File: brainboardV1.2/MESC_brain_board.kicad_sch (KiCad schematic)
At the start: 17 parts, among them J1 Conn_01x18, J2 Conn_01x04, Q1 my_BC337, U2 TJA1050T/CM,118, U2 Teensy4.0

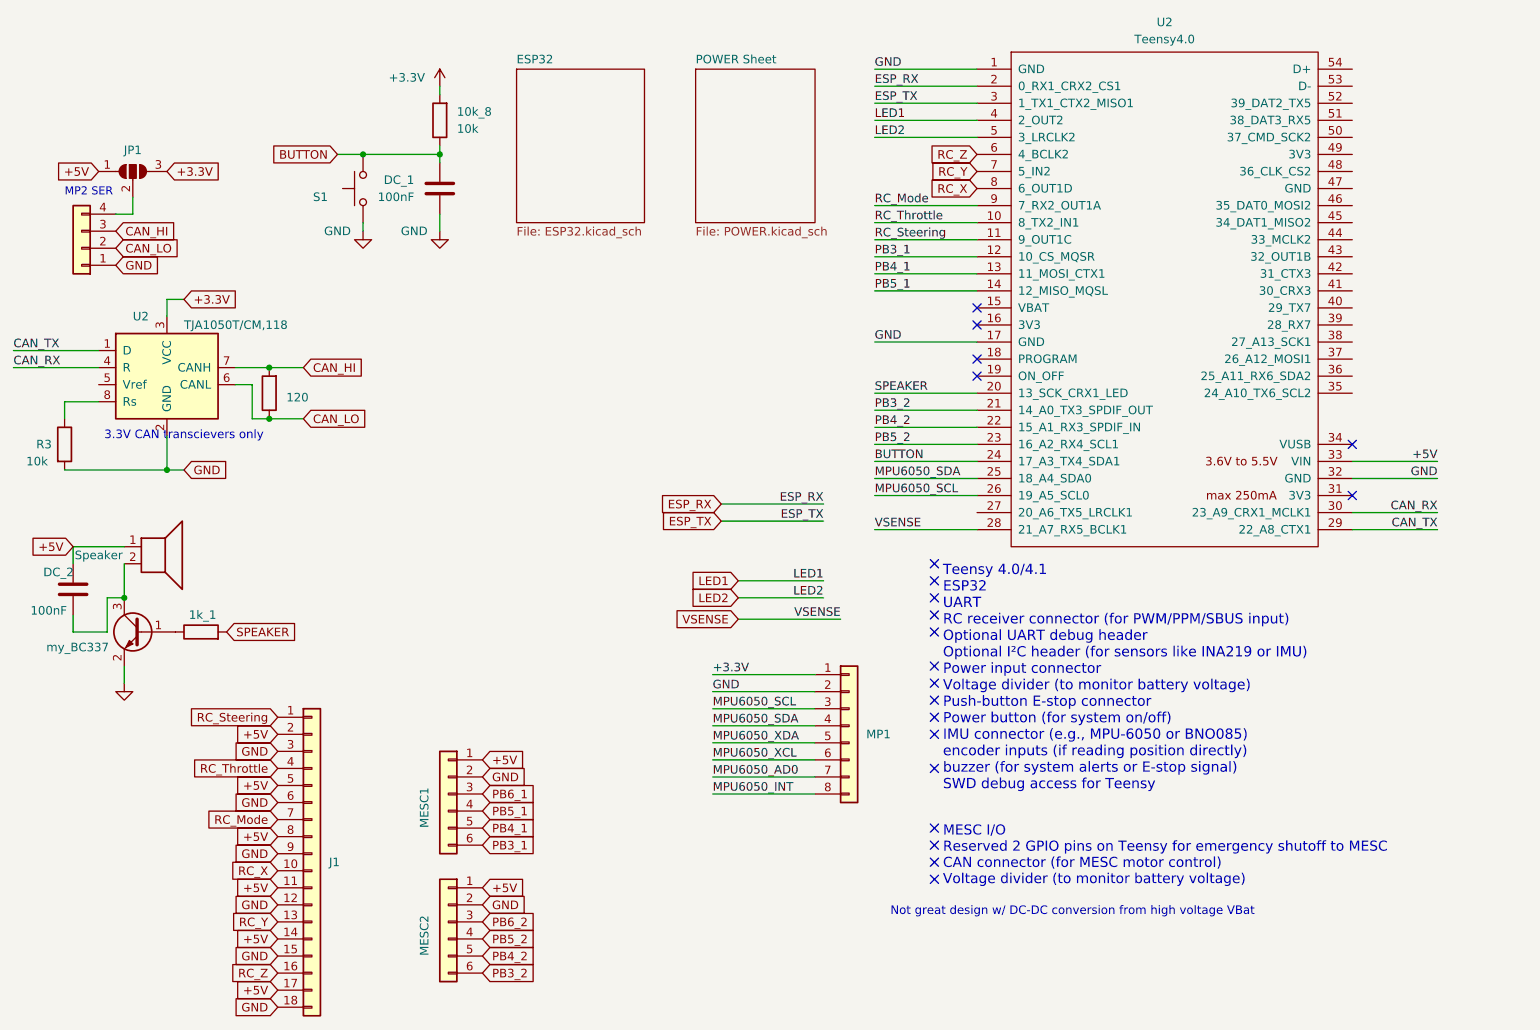
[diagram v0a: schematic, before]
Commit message: finalizing brain board v1.2
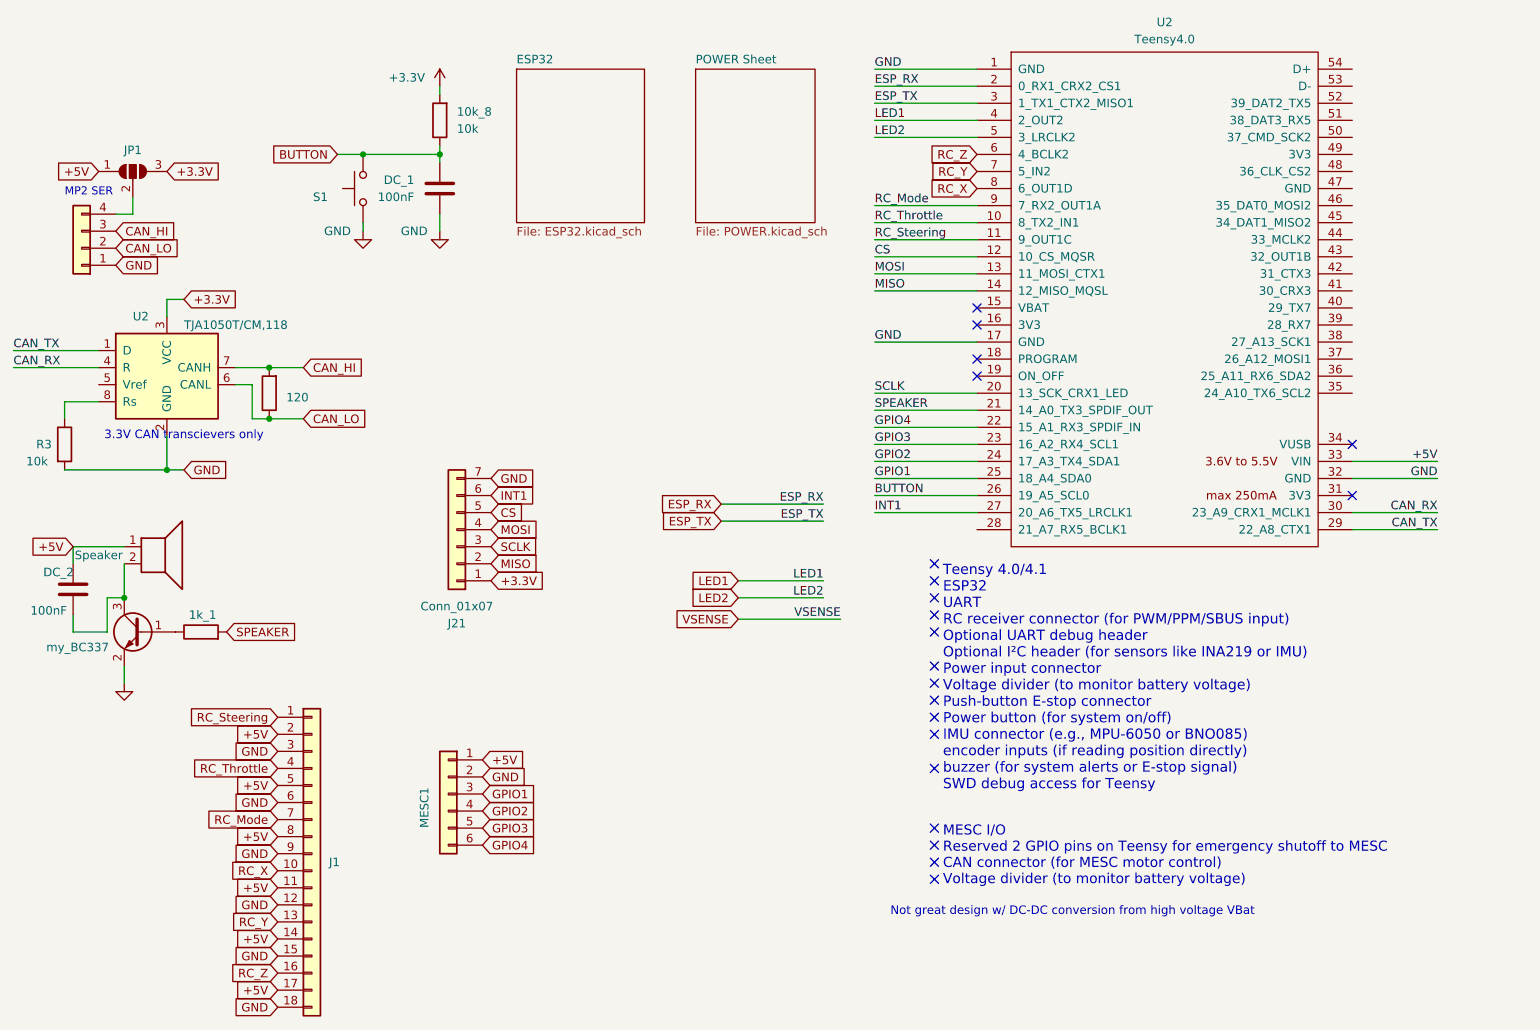
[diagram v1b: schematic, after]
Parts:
- removed MESC2: Conn_01x06, Connector_JST:JST_PH_B6B-PH-K_1x06_P2.00mm_Vertical, symbol Connector_Generic:Conn_01x06
- removed MP1: Conn_01x08, Connector_PinSocket_2.54mm:PinSocket_1x08_P2.54mm_Vertical, symbol Connector_Generic:Conn_01x08
- added J21: Conn_01x07, Connector_JST:JST_PH_B7B-PH-K_1x07_P2.00mm_Vertical, symbol Connector_Generic:Conn_01x07
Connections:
- net MPU6050_SCL is gone; now on net BUTTON: U2.26 (19_A5_SCL0)
- net PB3_2 is gone; now on net SPEAKER: U2.21 (14_A0_TX3_SPDIF_OUT)
- net PB5_2 is gone; now on net GPIO3: U2.23 (16_A2_RX4_SCL1)
- net PB6_1 is gone; now on net GPIO1: MESC1.3 (Pin_3)
- net +3.3V: now also J21.1 (Pin_1)
- net BUTTON: no longer U2.24 (17_A3_TX4_SDA1)
- net GND: now also J21.7 (Pin_7)
- net SPEAKER: no longer U2.20 (13_SCK_CRX1_LED)
- net VSENSE: no longer U2.28 (21_A7_RX5_BCLK1)
- net INT1: now reaches U2.27 (20_A6_TX5_LRCLK1)
- net INT1: now also J21.6 (Pin_6)
- net MPU6050_SDA renamed GPIO1
- net PB3_1 renamed CS
- net CS: now also J21.5 (Pin_5); no longer MESC1.6 (Pin_6)
- net PB4_1 renamed GPIO3
- net GPIO3: no longer U2.13 (11_MOSI_CTX1)
- net PB4_2 renamed GPIO4
- net GPIO4: now also MESC1.6 (Pin_6)
- net PB5_1 renamed GPIO2
- net GPIO2: now also U2.24 (17_A3_TX4_SDA1); no longer U2.14 (12_MISO_MQSL)
- new net MISO: J21.2 (Pin_2), U2.14 (12_MISO_MQSL)
- new net MOSI: J21.4 (Pin_4), U2.13 (11_MOSI_CTX1)
- new net SCLK: J21.3 (Pin_3), U2.20 (13_SCK_CRX1_LED)
